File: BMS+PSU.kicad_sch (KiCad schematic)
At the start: 2 parts, among them U9 BQ25601

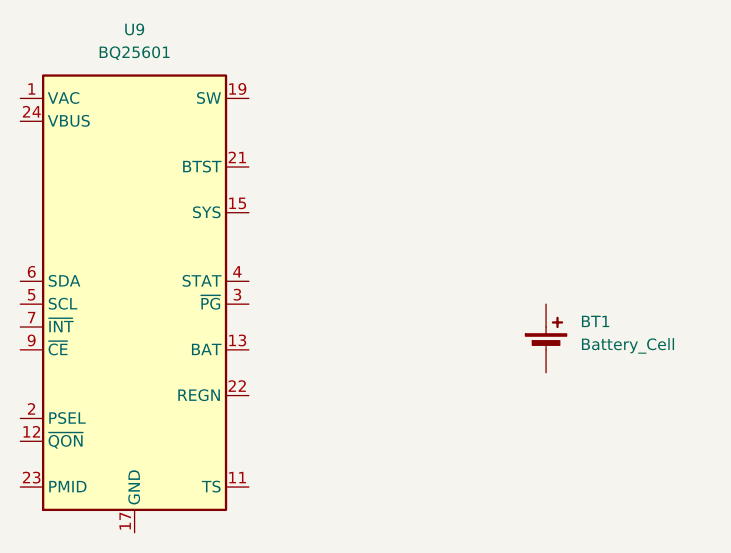
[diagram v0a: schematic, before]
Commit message: Backing up for productively workind during school tomorrow
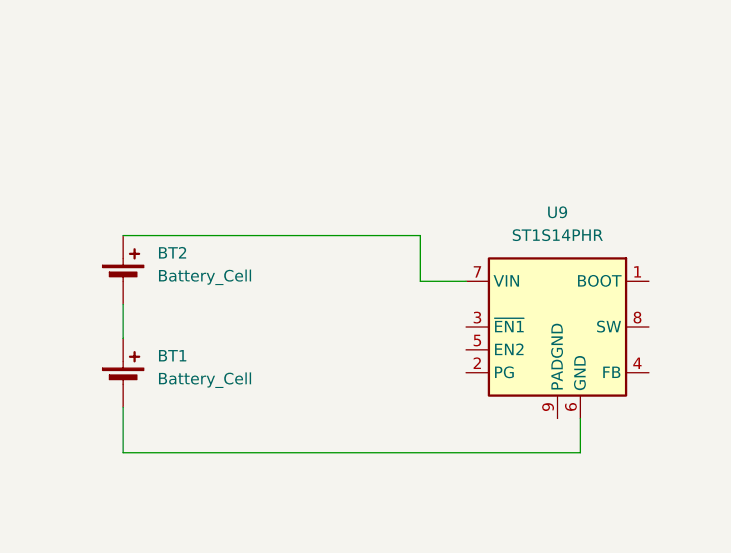
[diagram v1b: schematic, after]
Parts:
- removed U9: BQ25601, Package_DFN_QFN:Texas_S-PWQFN-N24_EP2.7x2.7mm_ThermalVias, symbol Battery_Management:BQ25601
- added BT2: Battery_Cell, symbol Device:Battery_Cell
- added U9: ST1S14PHR, Package_SO:TI_SO-PowerPAD-8, symbol Regulator_Switching:ST1S14PHR
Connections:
- net at BT1.1 (+): now also BT2.2 (-)
- net at BT1.2 (-): now also U9.6 (GND)
- new net: BT2.1 (+), U9.7 (VIN)
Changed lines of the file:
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@@
 (kicad_sch (version 20230121) (generator eeschema)
   (paper "A4")
-  (symbol (lib_id "Battery_Management:BQ25601") (at 134.62 96.52 0) (unit 1)
+  (wire (pts (xy 133.35 88.9) (xy 166.37 88.9))
+    (stroke (width 0) (type default))
+  )
+  (wire (pts (xy 133.35 113.03) (xy 184.15 113.03))
+    (stroke (width 0) (type default))
+  )
+  (wire (pts (xy 184.15 113.03) (xy 184.15 109.22))
+    (stroke (width 0) (type default))
+  )
+  (wire (pts (xy 133.35 107.95) (xy 133.35 113.03))
+    (stroke (width 0) (type default))
+  )
+  (wire (pts (xy 133.35 96.52) (xy 133.35 100.33))
+    (stroke (width 0) (type default))
+  )
+  (wire (pts (xy 166.37 93.98) (xy 171.45 93.98))
+    (stroke (width 0) (type default))
+  )
+  (wire (pts (xy 166.37 88.9) (xy 166.37 93.98))
+    (stroke (width 0) (type default))
+  )
+  (symbol (lib_id "Regulator_Switching:ST1S14PHR") (at 181.61 99.06 0) (unit 1)
     (in_bom yes) (on_board yes) (dnp no) (fields_autoplaced)
-    (property "Reference" "U9" (at 134.62 66.04 0)
+    (property "Reference" "U9" (at 181.61 86.36 0)
       (effects (font (size 1.27 1.27)))
     )
-    (property "Value" "BQ25601" (at 134.62 68.58 0)
+    (property "Value" "ST1S14PHR" (at 181.61 88.9 0)
       (effects (font (size 1.27 1.27)))
     )
-    (property "Footprint" "Package_DFN_QFN:Texas_S-PWQFN-N24_EP2.7x2.7mm_ThermalVias" (at 134.62 67.31 0)
+    (property "Footprint" "Package_SO:TI_SO-PowerPAD-8" (at 184.785 107.95 0)
+      (effects (font (size 1.27 1.27) italic) (justify left) hide)
+    )
+    (property "Datasheet" "http://www.st.com/internet/com/TECHNICAL_RESOURCES/TECHNICAL_LITERATURE/DATASHEET/CD00285678.pdf" (at 181.61 99.06 0)
       (effects (font (size 1.27 1.27)) hide)
     )
-    (property "Datasheet" "http://www.ti.com/lit/ds/symlink/bq25601.pdf" (at 134.62 60.96 0)
-      (effects (font (size 1.27 1.27)) hide)
-    )
-    (pin "22")
+    (pin "5")
+    (pin "6")
+    (pin "4")
+    (pin "2")
+    (pin "1")
     (pin "7")
     (pin "3")
-    (pin "5")
-    (pin "17")
-    (pin "1")
-    (pin "16")
     (pin "8")
-    (pin "13")
-    (pin "12")
-    (pin "11")
-    (pin "10")
-    (pin "14")
-    (pin "15")
-    (pin "6")
     (pin "9")
-    (pin "21")
-    (pin "19")
-    (pin "24")
-    (pin "4")
-    (pin "2")
-    (pin "23")
-    (pin "18")
-    (pin "20")
-    (pin "25")
     (instances
       (project "Flight-Computer"
@@
     )
   )
-  (symbol (lib_id "Device:Battery_Cell") (at 180.34 101.6 0) (unit 1)
+  (symbol (lib_id "Device:Battery_Cell") (at 133.35 93.98 0) (unit 1)
     (in_bom yes) (on_board yes) (dnp no) (fields_autoplaced)
-    (property "Reference" "BT1" (at 184.15 98.4885 0)
+    (property "Reference" "BT2" (at 137.16 90.8685 0)
       (effects (font (size 1.27 1.27)) (justify left))
     )
-    (property "Value" "Battery_Cell" (at 184.15 101.0285 0)
+    (property "Value" "Battery_Cell" (at 137.16 93.4085 0)
       (effects (font (size 1.27 1.27)) (justify left))
     )
-    (property "Footprint" "" (at 180.34 100.076 90)
+    (property "Footprint" "" (at 133.35 92.456 90)
       (effects (font (size 1.27 1.27)) hide)
     )
-    (property "Datasheet" "~" (at 180.34 100.076 90)
+    (property "Datasheet" "~" (at 133.35 92.456 90)
       (effects (font (size 1.27 1.27)) hide)
     )
+    (pin "2")
+    (pin "1")
+    (instances
+      (project "Flight-Computer"
+        (path "/3ff93668-efc3-42e6-a72e-521229bcc4c8/caf9fb23-904f-4f5d-9408-b4ebadda3c1c"
+          (reference "BT2") (unit 1)
+        )
+      )
+    )
+  )
+  (symbol (lib_id "Device:Battery_Cell") (at 133.35 105.41 0) (unit 1)
+    (in_bom yes) (on_board yes) (dnp no) (fields_autoplaced)
+    (property "Reference" "BT1" (at 137.16 102.2985 0)
+      (effects (font (size 1.27 1.27)) (justify left))
+    )
+    (property "Value" "Battery_Cell" (at 137.16 104.8385 0)
+      (effects (font (size 1.27 1.27)) (justify left))
+    )
+    (property "Footprint" "" (at 133.35 103.886 90)
+      (effects (font (size 1.27 1.27)) hide)
+    )
+    (property "Datasheet" "~" (at 133.35 103.886 90)
+      (effects (font (size 1.27 1.27)) hide)
+    )
